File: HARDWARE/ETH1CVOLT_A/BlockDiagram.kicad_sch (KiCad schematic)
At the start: 4 parts

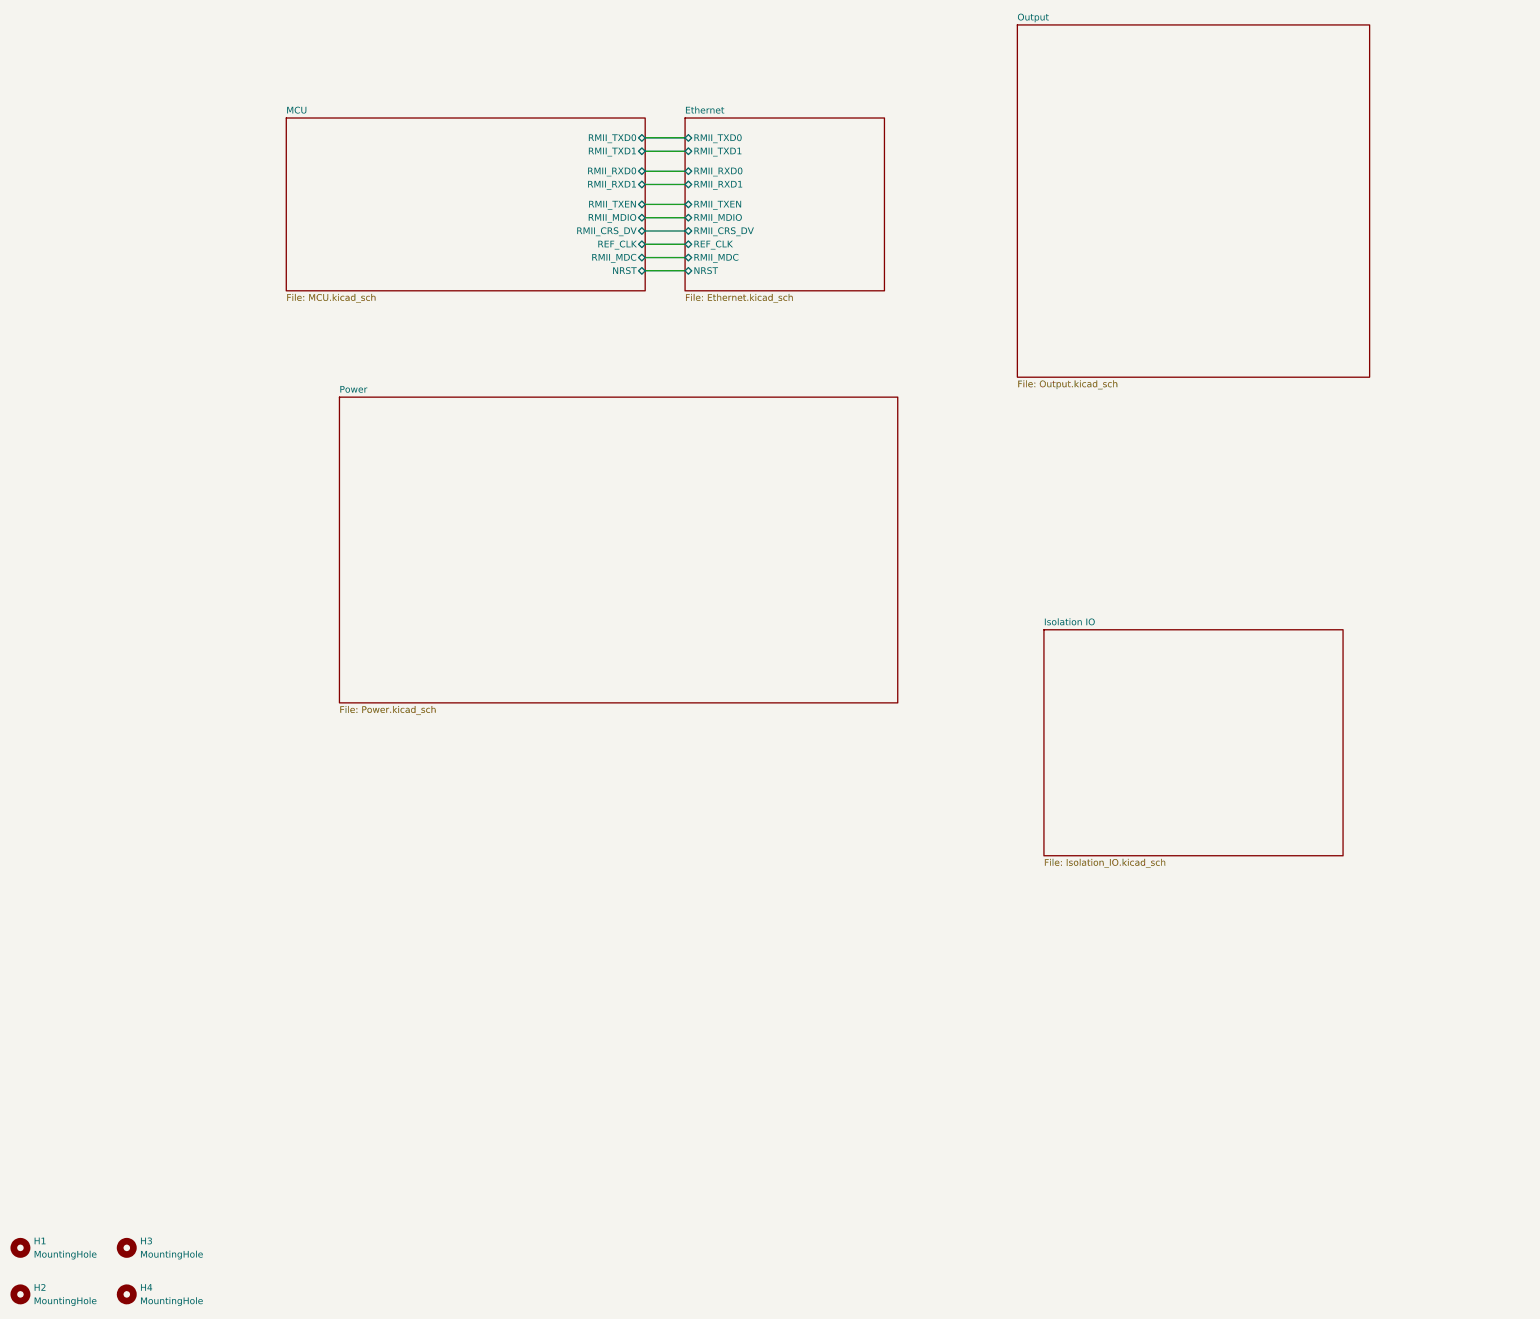
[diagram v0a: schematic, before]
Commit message: Development
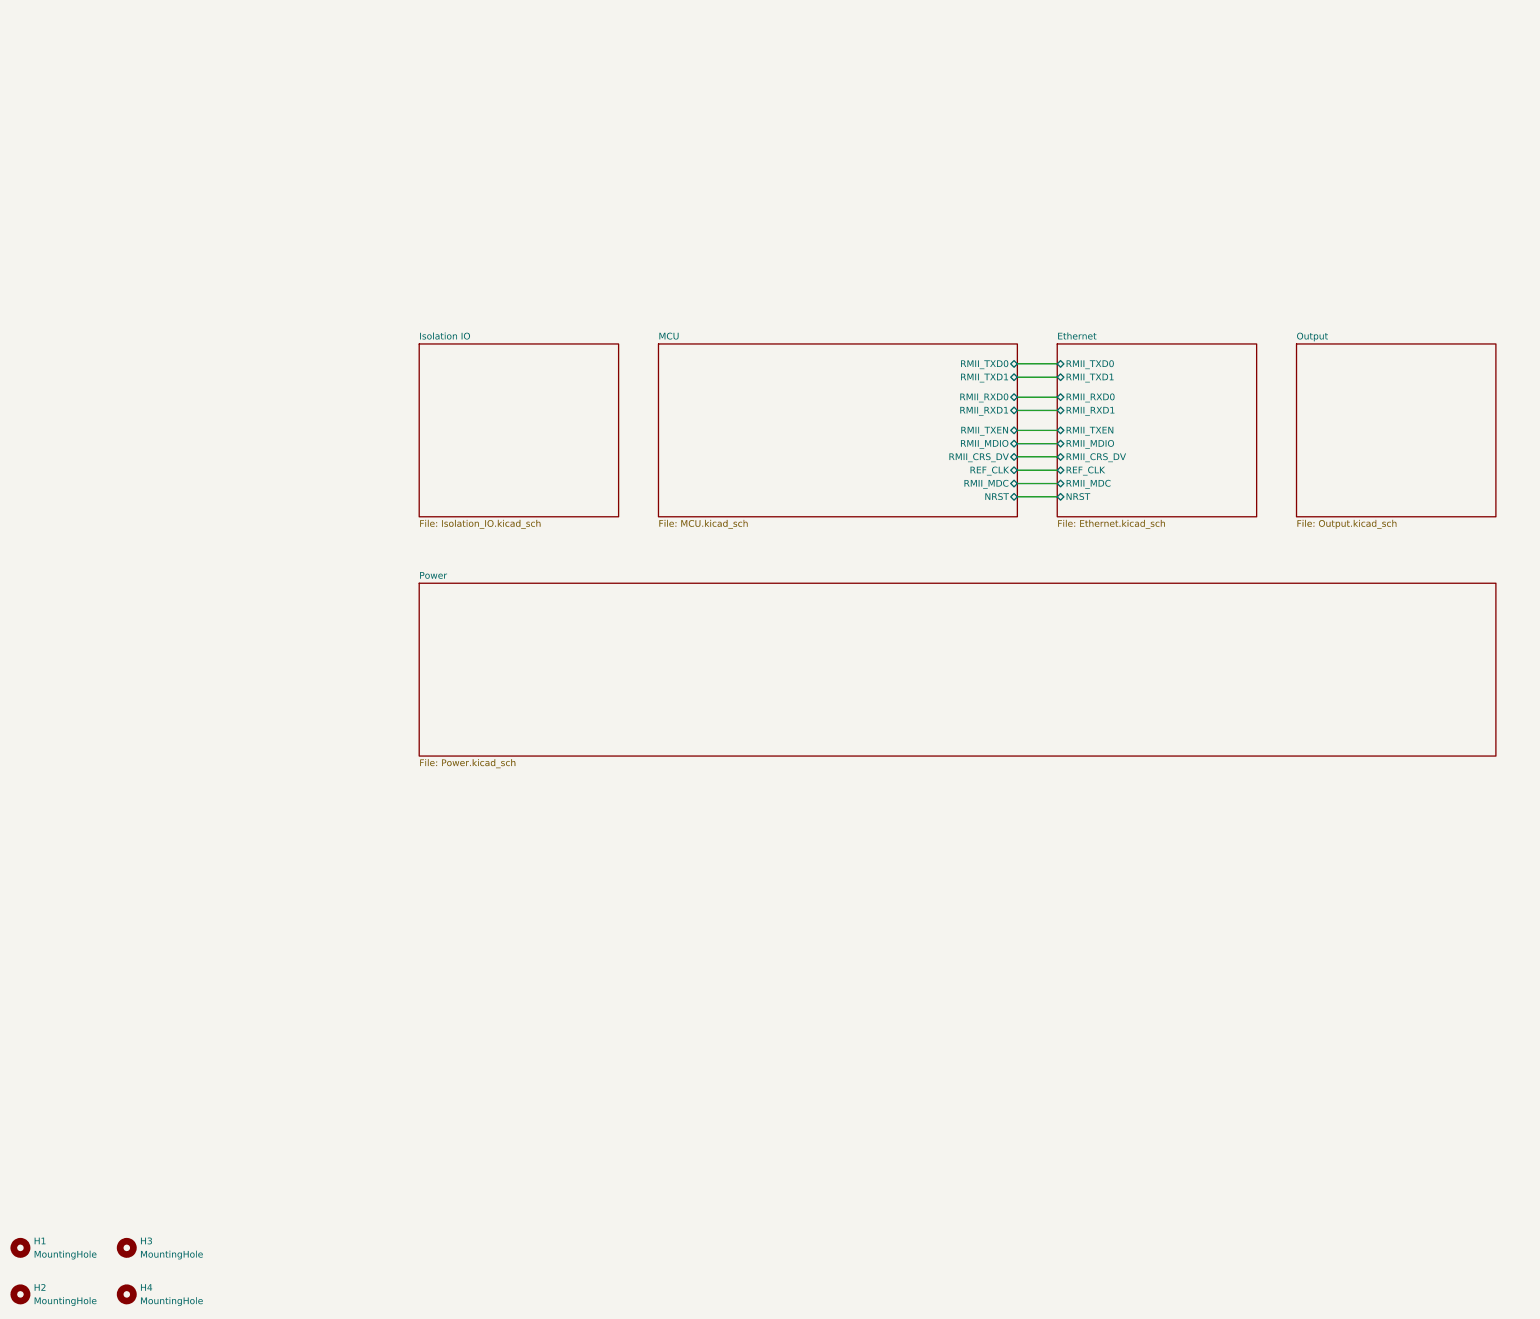
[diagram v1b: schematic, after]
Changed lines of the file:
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@@
 	(wire
 		(pts
-			(xy 144.78 54.61) (xy 152.4 54.61)
-		)
-		(stroke
-			(width 0)
-			(type default)
-		)
-	)
-	(wire
-		(pts
-			(xy 144.78 63.5) (xy 152.4 63.5)
-		)
-		(stroke
-			(width 0)
-			(type default)
-		)
-	)
-	(wire
-		(pts
-			(xy 144.78 69.85) (xy 152.4 69.85)
-		)
-		(stroke
-			(width 0)
-			(type default)
-		)
-	)
-	(wire
-		(pts
-			(xy 144.78 72.39) (xy 152.4 72.39)
-		)
-		(stroke
-			(width 0)
-			(type default)
-		)
-	)
-	(wire
-		(pts
-			(xy 144.78 74.93) (xy 152.4 74.93)
-		)
-		(stroke
-			(width 0)
-			(type default)
-		)
-	)
-	(wire
-		(pts
-			(xy 144.78 60.96) (xy 152.4 60.96)
-		)
-		(stroke
-			(width 0)
-			(type default)
-		)
-	)
-	(wire
-		(pts
-			(xy 144.78 80.01) (xy 152.4 80.01)
-		)
-		(stroke
-			(width 0)
-			(type default)
-		)
-	)
-	(wire
-		(pts
-			(xy 144.78 67.31) (xy 152.4 67.31)
-		)
-		(stroke
-			(width 0)
-			(type default)
-		)
-	)
-	(wire
-		(pts
-			(xy 144.78 57.15) (xy 152.4 57.15)
-		)
-		(stroke
-			(width 0)
-			(type default)
-		)
-	)
-	(wire
-		(pts
-			(xy 144.78 77.47) (xy 152.4 77.47)
+			(xy 215.9 97.79) (xy 223.52 97.79)
+		)
+		(stroke
+			(width 0)
+			(type default)
+		)
+	)
+	(wire
+		(pts
+			(xy 215.9 106.68) (xy 223.52 106.68)
+		)
+		(stroke
+			(width 0)
+			(type default)
+		)
+	)
+	(wire
+		(pts
+			(xy 215.9 113.03) (xy 223.52 113.03)
+		)
+		(stroke
+			(width 0)
+			(type default)
+		)
+	)
+	(wire
+		(pts
+			(xy 215.9 115.57) (xy 223.52 115.57)
+		)
+		(stroke
+			(width 0)
+			(type default)
+		)
+	)
+	(wire
+		(pts
+			(xy 215.9 118.11) (xy 223.52 118.11)
+		)
+		(stroke
+			(width 0)
+			(type default)
+		)
+	)
+	(wire
+		(pts
+			(xy 215.9 104.14) (xy 223.52 104.14)
+		)
+		(stroke
+			(width 0)
+			(type default)
+		)
+	)
+	(wire
+		(pts
+			(xy 215.9 123.19) (xy 223.52 123.19)
+		)
+		(stroke
+			(width 0)
+			(type default)
+		)
+	)
+	(wire
+		(pts
+			(xy 215.9 110.49) (xy 223.52 110.49)
+		)
+		(stroke
+			(width 0)
+			(type default)
+		)
+	)
+	(wire
+		(pts
+			(xy 215.9 100.33) (xy 223.52 100.33)
+		)
+		(stroke
+			(width 0)
+			(type default)
+		)
+	)
+	(wire
+		(pts
+			(xy 215.9 120.65) (xy 223.52 120.65)
 		)
 		(stroke
@@
 	)
 	(sheet
-		(at 86.36 104.14)
-		(size 106.68 58.42)
+		(at 101.6 139.7)
+		(size 205.74 33.02)
 		(exclude_from_sim no)
 		(in_bom yes)
@@
 		)
 		(property "Sheetname" "Power"
-			(at 86.36 103.4284 0)
+			(at 101.6 138.9884 0)
 			(effects
 				(font
@@
 		)
 		(property "Sheetfile" "Power.kicad_sch"
-			(at 86.36 163.1446 0)
+			(at 101.6 173.3046 0)
 			(effects
 				(font
@@
 	)
 	(sheet
-		(at 220.98 148.59)
-		(size 57.15 43.18)
+		(at 101.6 93.98)
+		(size 38.1 33.02)
 		(exclude_from_sim no)
 		(in_bom yes)
@@
 		)
 		(property "Sheetname" "Isolation IO"
-			(at 220.98 147.8784 0)
+			(at 101.6 93.2684 0)
 			(effects
 				(font
@@
 		)
 		(property "Sheetfile" "Isolation_IO.kicad_sch"
-			(at 220.98 192.3546 0)
+			(at 101.6 127.5846 0)
 			(effects
 				(font
@@
 	)
 	(sheet
-		(at 215.9 33.02)
-		(size 67.31 67.31)
+		(at 269.24 93.98)
+		(size 38.1 33.02)
 		(exclude_from_sim no)
 		(in_bom yes)
@@
 		)
 		(property "Sheetname" "Output"
-			(at 215.9 32.3084 0)
+			(at 269.24 93.2684 0)
 			(effects
 				(font
@@
 		)
 		(property "Sheetfile" "Output.kicad_sch"
-			(at 215.9 100.9146 0)
+			(at 269.24 127.5846 0)
 			(effects
 				(font
@@
 	)
 	(sheet
-		(at 152.4 50.8)
+		(at 223.52 93.98)
 		(size 38.1 33.02)
 		(exclude_from_sim no)
@@
 		)
 		(property "Sheetname" "Ethernet"
-			(at 152.4 50.0884 0)
+			(at 223.52 93.2684 0)
 			(effects
 				(font
@@
 		)
 		(property "Sheetfile" "Ethernet.kicad_sch"
-			(at 152.4 84.4046 0)
+			(at 223.52 127.5846 0)
 			(effects
 				(font
@@
 		)
 		(pin "RMII_TXD1" bidirectional
-			(at 152.4 57.15 180)
+			(at 223.52 100.33 180)
 			(effects
 				(font
@@
 		)
 		(pin "REF_CLK" bidirectional
-			(at 152.4 74.93 180)
+			(at 223.52 118.11 180)
 			(effects
 				(font
@@
 		)
 		(pin "RMII_MDIO" bidirectional
-			(at 152.4 69.85 180)
+			(at 223.52 113.03 180)
 			(effects
 				(font
@@
 		)
 		(pin "RMII_CRS_DV" bidirectional
-			(at 152.4 72.39 180)
+			(at 223.52 115.57 180)
 			(effects
 				(font
@@
 		)
 		(pin "RMII_RXD1" bidirectional
-			(at 152.4 63.5 180)
+			(at 223.52 106.68 180)
 			(effects
 				(font
@@
 		)
 		(pin "RMII_MDC" bidirectional
-			(at 152.4 77.47 180)
+			(at 223.52 120.65 180)
 			(effects
 				(font
@@
 		)
 		(pin "RMII_TXD0" bidirectional
-			(at 152.4 54.61 180)
+			(at 223.52 97.79 180)
 			(effects
 				(font
@@
 		)
 		(pin "RMII_TXEN" bidirectional
-			(at 152.4 67.31 180)
+			(at 223.52 110.49 180)
 			(effects
 				(font
@@
 		)
 		(pin "NRST" bidirectional
-			(at 152.4 80.01 180)
+			(at 223.52 123.19 180)
 			(effects
 				(font
@@
 		)
 		(pin "RMII_RXD0" bidirectional
-			(at 152.4 60.96 180)
+			(at 223.52 104.14 180)
 			(effects
 				(font
@@
 	)
 	(sheet
-		(at 76.2 50.8)
+		(at 147.32 93.98)
 		(size 68.58 33.02)
 		(exclude_from_sim no)
@@
 		)
 		(property "Sheetname" "MCU"
-			(at 76.2 50.0884 0)
+			(at 147.32 93.2684 0)
 			(effects
 				(font
@@
 		)
 		(property "Sheetfile" "MCU.kicad_sch"
-			(at 76.2 84.4046 0)
+			(at 147.32 127.5846 0)
 			(effects
 				(font
@@
 		)
 		(pin "RMII_MDC" bidirectional
-			(at 144.78 77.47 0)
+			(at 215.9 120.65 0)
 			(effects
 				(font
@@
 		)
 		(pin "RMII_MDIO" bidirectional
-			(at 144.78 69.85 0)
+			(at 215.9 113.03 0)
 			(effects
 				(font
@@
 		)
 		(pin "RMII_TXD1" bidirectional
-			(at 144.78 57.15 0)
+			(at 215.9 100.33 0)
 			(effects
 				(font
@@
 		)
 		(pin "REF_CLK" bidirectional
-			(at 144.78 74.93 0)
+			(at 215.9 118.11 0)
 			(effects
 				(font
@@
 		)
 		(pin "RMII_TXEN" bidirectional
-			(at 144.78 67.31 0)
+			(at 215.9 110.49 0)
 			(effects
 				(font
@@
 		)
 		(pin "RMII_TXD0" bidirectional
-			(at 144.78 54.61 0)
+			(at 215.9 97.79 0)
 			(effects
 				(font
@@
 		)
 		(pin "NRST" bidirectional
-			(at 144.78 80.01 0)
+			(at 215.9 123.19 0)
 			(effects
 				(font
@@
 		)
 		(pin "RMII_CRS_DV" bidirectional
-			(at 144.78 72.39 0)
+			(at 215.9 115.57 0)
 			(effects
 				(font
@@
 		)
 		(pin "RMII_RXD0" bidirectional
-			(at 144.78 60.96 0)
+			(at 215.9 104.14 0)
 			(effects
 				(font
@@
 		)
 		(pin "RMII_RXD1" bidirectional
-			(at 144.78 63.5 0)
-			(effects
-				(font
+			(at 215.9 106.68 0)
+			(effects
+				(font

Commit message: Development
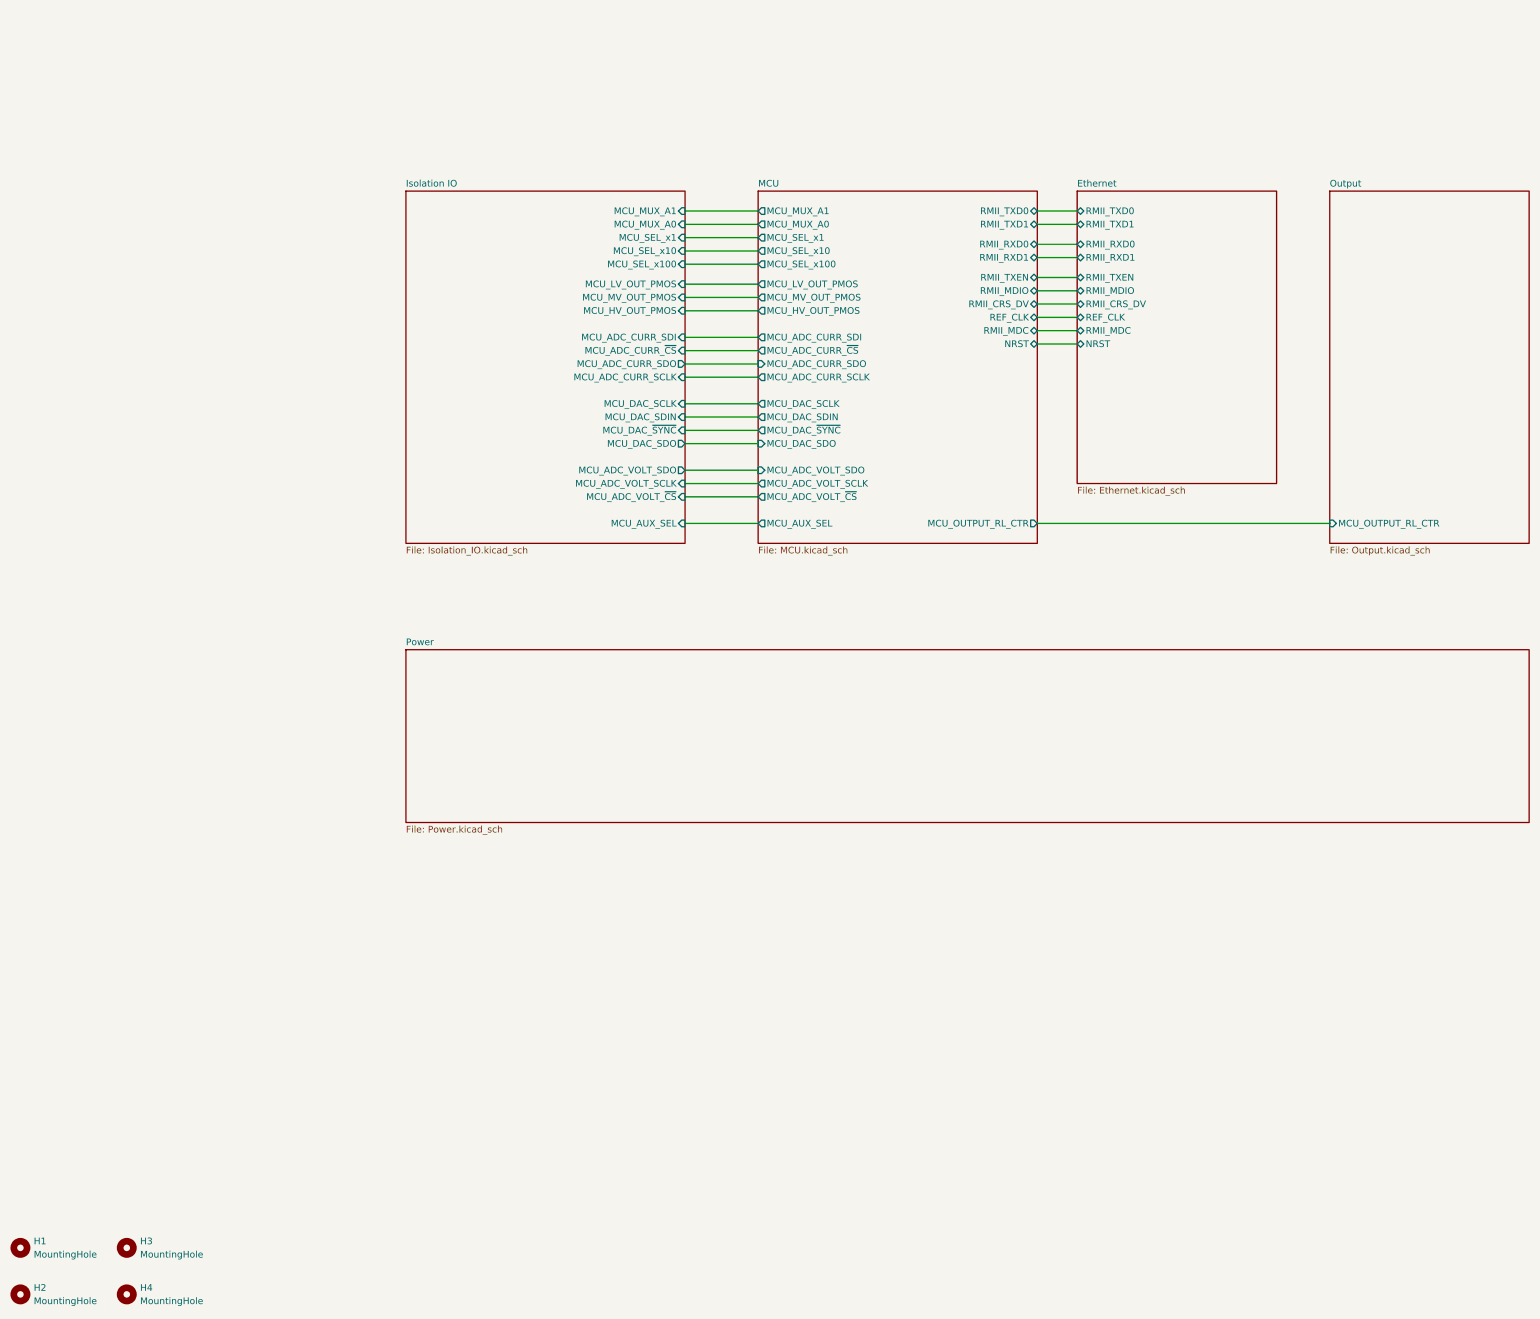
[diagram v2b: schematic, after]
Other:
- sheet Isolation IO ports: added MCU_ADC_CURR_SCLK, MCU_ADC_CURR_SDI, MCU_ADC_CURR_SDO, MCU_ADC_CURR_~{CS}, MCU_ADC_VOLT_SCLK, MCU_ADC_VOLT_SDO, MCU_ADC_VOLT_~{CS}, MCU_AUX_SEL, MCU_DAC_SCLK, MCU_DAC_SDIN, MCU_DAC_SDO, MCU_DAC_~{SYNC}, MCU_HV_OUT_PMOS, MCU_LV_OUT_PMOS, MCU_MUX_A0, MCU_MUX_A1, MCU_MV_OUT_PMOS, MCU_SEL_x1, MCU_SEL_x10, MCU_SEL_x100; removed none
- sheet MCU ports: added MCU_ADC_CURR_SCLK, MCU_ADC_CURR_SDI, MCU_ADC_CURR_SDO, MCU_ADC_CURR_~{CS}, MCU_ADC_VOLT_SCLK, MCU_ADC_VOLT_SDO, MCU_ADC_VOLT_~{CS}, MCU_AUX_SEL, MCU_DAC_SCLK, MCU_DAC_SDIN, MCU_DAC_SDO, MCU_DAC_~{SYNC}, MCU_HV_OUT_PMOS, MCU_LV_OUT_PMOS, MCU_MUX_A0, MCU_MUX_A1, MCU_MV_OUT_PMOS, MCU_OUTPUT_RL_CTR, MCU_SEL_x1, MCU_SEL_x10, MCU_SEL_x100; removed none
- sheet Output ports: added MCU_OUTPUT_RL_CTR; removed none
